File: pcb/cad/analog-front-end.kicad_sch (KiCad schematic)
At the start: 48 parts, among them J201 Conn_Coaxial, U201 OPA2227, U202 AMC1200, U203 AD8421, U204 LM393-N

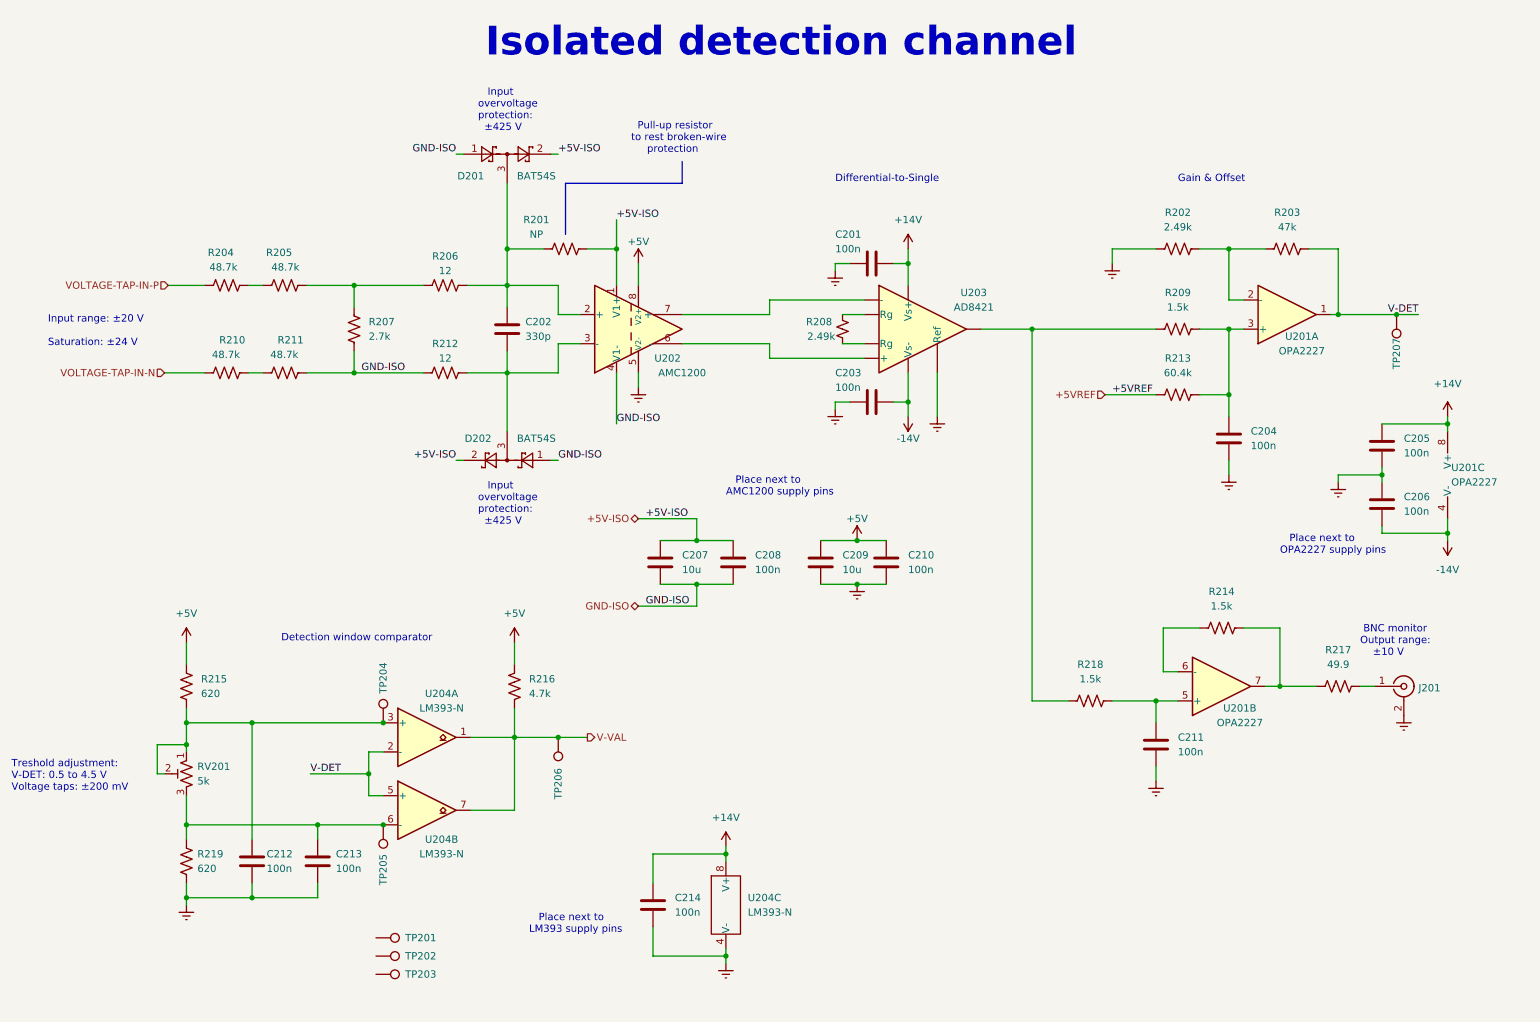
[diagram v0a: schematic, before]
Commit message: Include resistors tied to +5V and GND in isolated front-end circuits
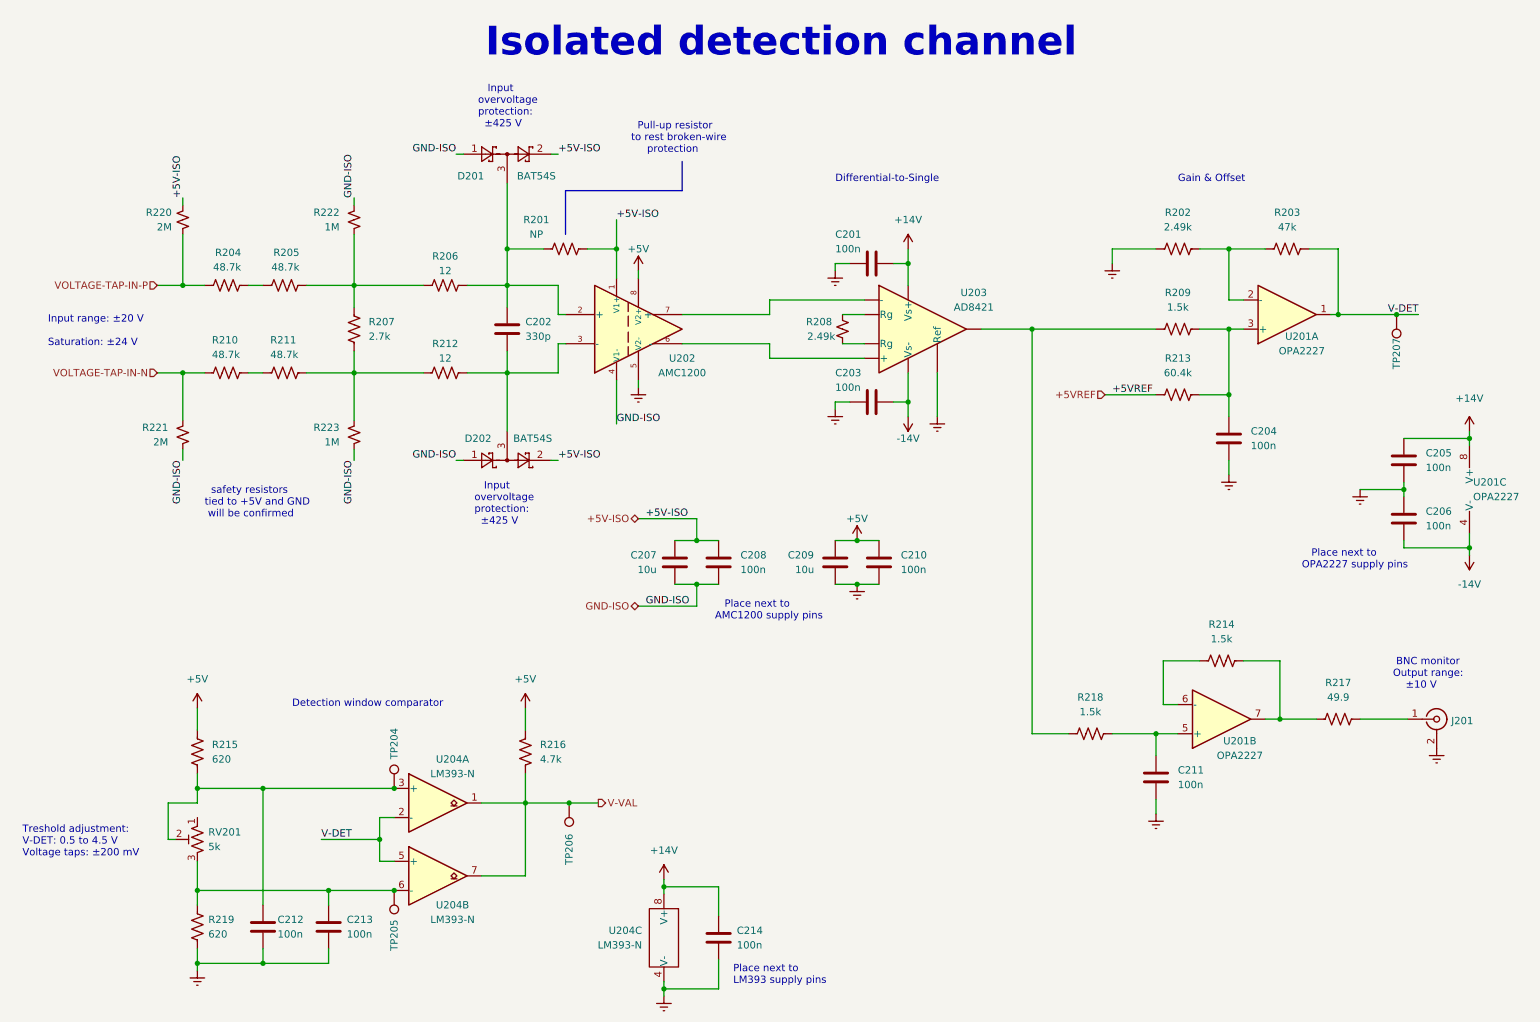
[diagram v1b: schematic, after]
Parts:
- removed TP201, TP202, TP203: TestPoint, symbol Connector:TestPoint
- added R220, R221: 2M, Resistor_SMD:R_0805_2012Metric_Pad1.20x1.40mm_HandSolder, symbol Device:R_Small_US
- added R222, R223: 1M, Resistor_SMD:R_0805_2012Metric_Pad1.20x1.40mm_HandSolder, symbol Device:R_Small_US
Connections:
- net +5V-ISO: now also R220.2
- net GND-ISO: now also R221.1, R222.2, R223.1; no longer R207.2, R211.2, R212.1
- net VOLTAGE-TAP-IN-N: now also R221.2
- net VOLTAGE-TAP-IN-P: now also R220.1
- net at R205.2, R206.1, R207.1: now also R222.1
- net at C212.1, R215.1, RV201.2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: no longer RV201.1
- new net: R207.2, R211.2, R212.1, R223.2
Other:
- note added: "safety resistors tied to +5V and GND will be confirmed"
- moved on the sheet: C205, C206, C207, C208, C209, C210, C211, C212, C213, C214, D202, J201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

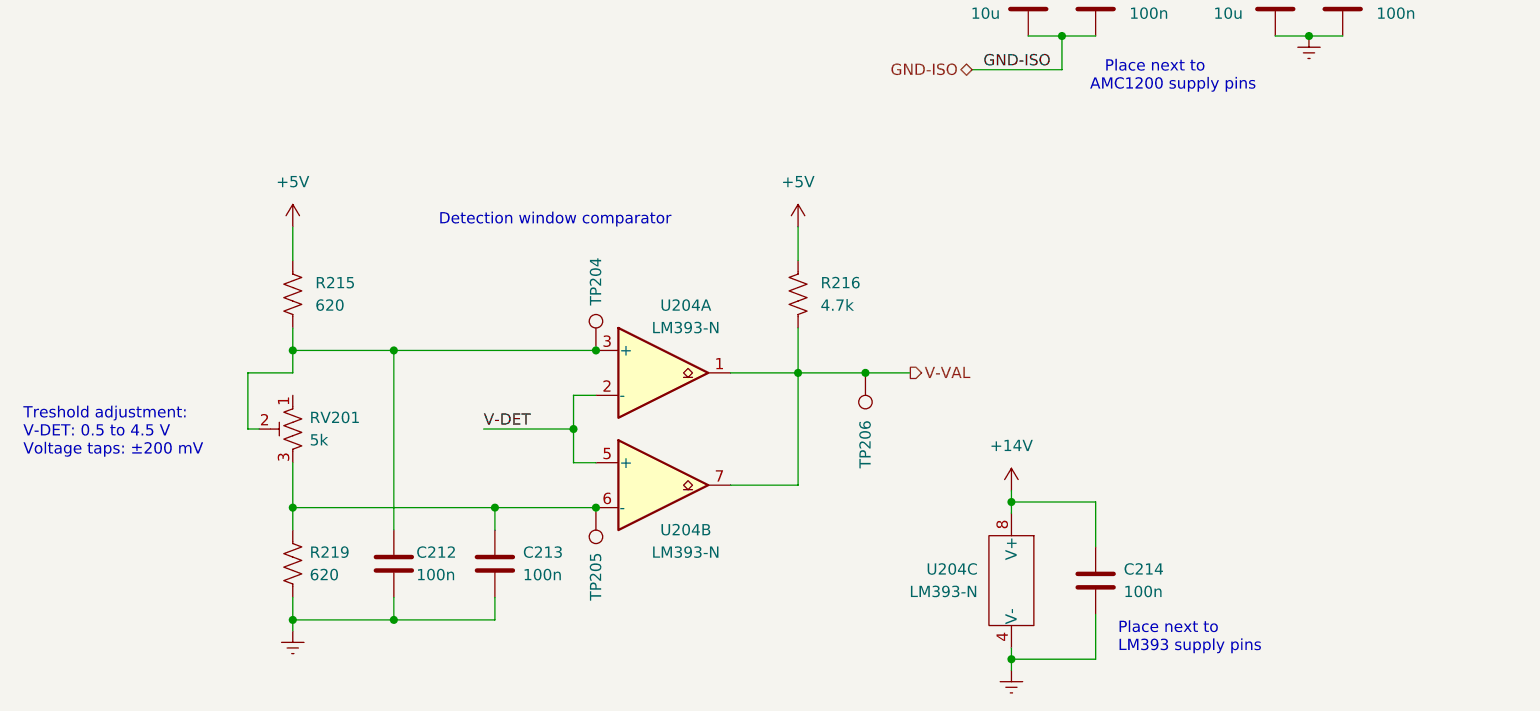
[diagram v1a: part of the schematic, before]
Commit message: Improve window comparator, +5V-REF and relay driver circuits close #19 close #20 close #22
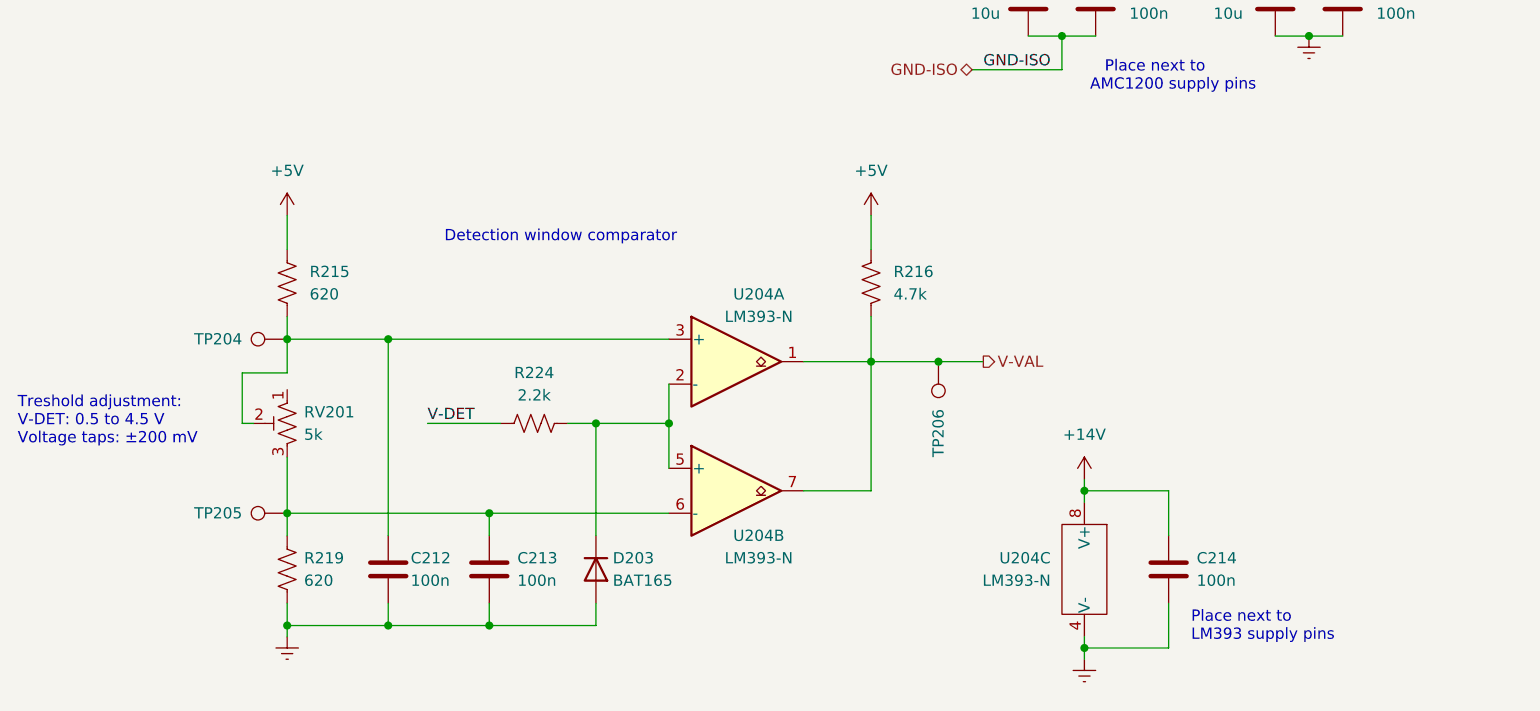
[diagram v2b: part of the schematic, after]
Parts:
- added D203: BAT165, Diode_SMD:D_SOD-323_HandSoldering, symbol Device:D
- added R224: 2.2k, Resistor_SMD:R_0805_2012Metric_Pad1.20x1.40mm_HandSolder, symbol Device:R_US
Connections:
- net Earth: now also D203.2 (A)
- net V-DET: now also R224.1; no longer U204.2 (-), U204.5 (+)
- new net: D203.1 (K), R224.2, U204.2 (-), U204.5 (+)
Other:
- moved on the sheet: C212, C213, C214, R215, R216, R219, RV201, TP204, TP205, TP206, U204A, U204B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
